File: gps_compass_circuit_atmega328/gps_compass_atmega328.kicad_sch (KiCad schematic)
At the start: 3 parts, among them U3 ATmega328P-A

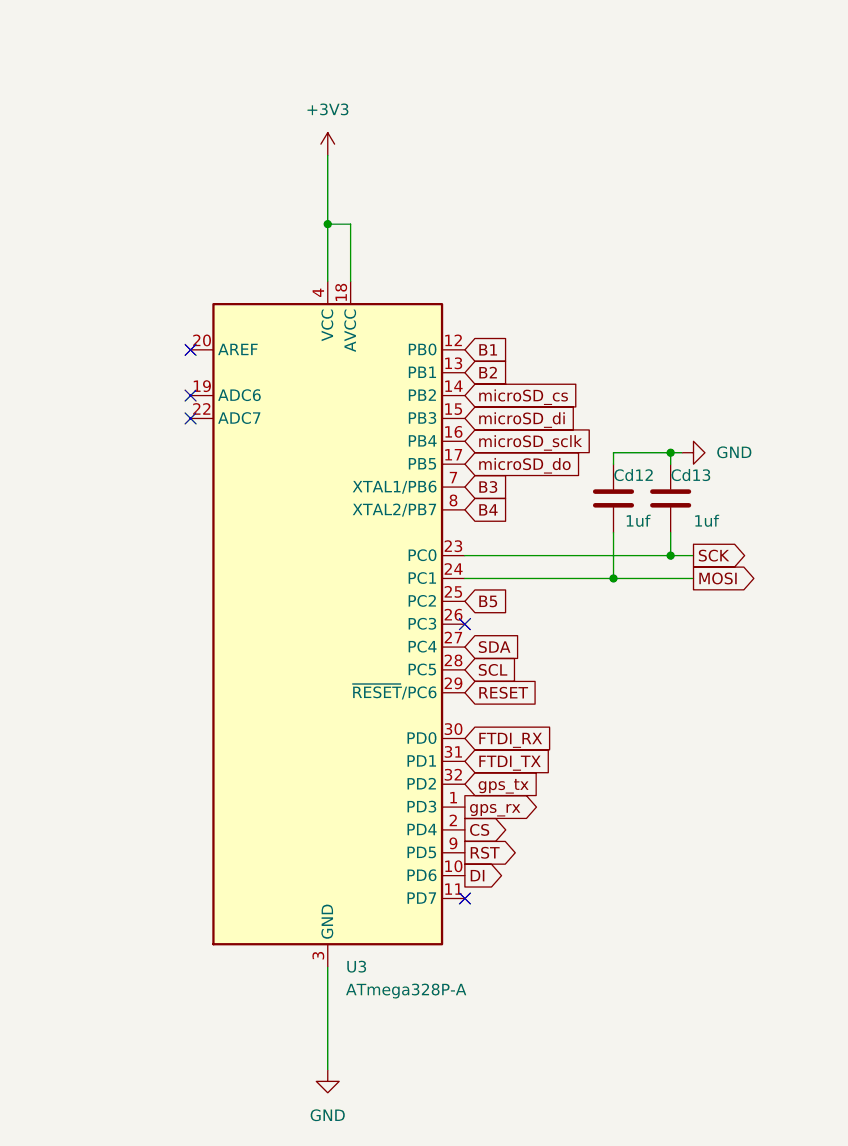
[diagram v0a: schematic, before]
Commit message: upd circuit
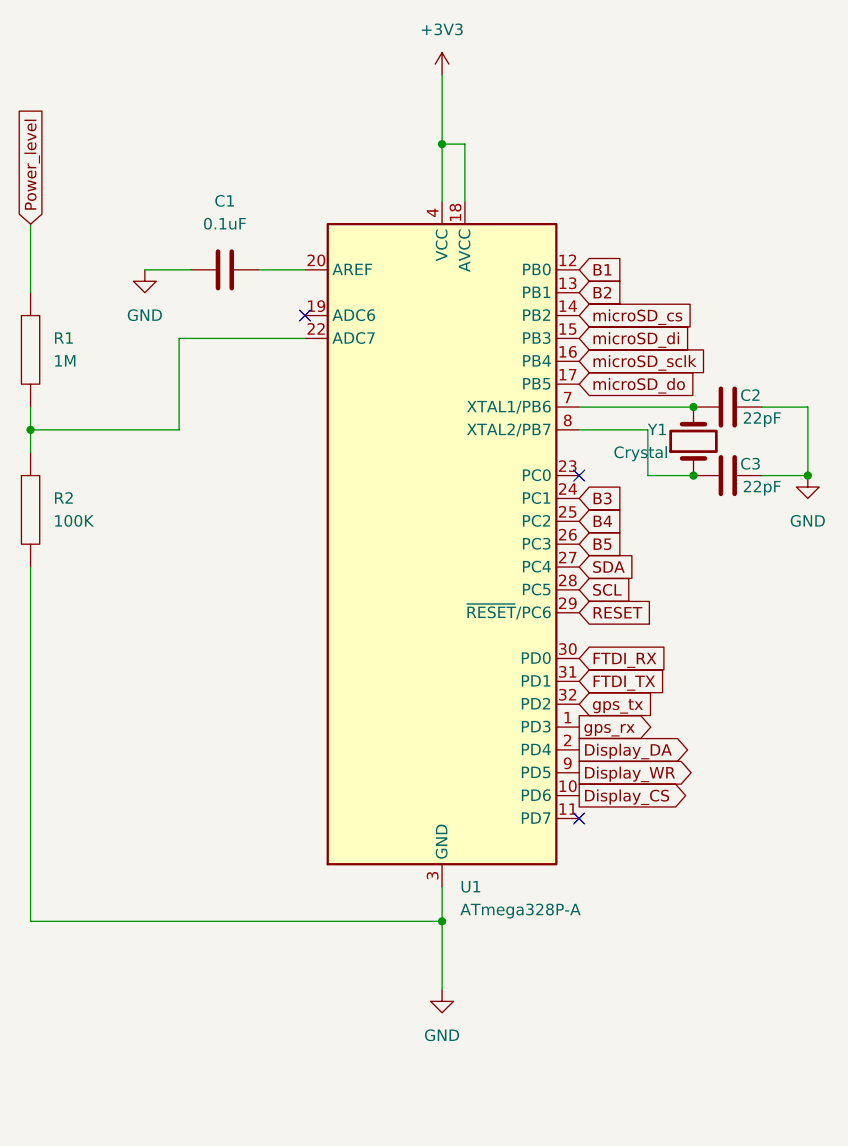
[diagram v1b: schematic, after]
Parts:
- removed Cd12, Cd13: 1uf, Capacitor_SMD:C_0603_1608Metric, symbol Device:C
- removed U3: ATmega328P-A, Package_QFP:TQFP-32_7x7mm_P0.8mm, symbol MCU_Microchip_ATmega:ATmega328P-A
- added C1: 0.1uF, Capacitor_SMD:C_0603_1608Metric, symbol Device:C
- added C2, C3: 22pF, Capacitor_SMD:C_0603_1608Metric, symbol Device:C
- added R1: 1M, Capacitor_SMD:C_0603_1608Metric, symbol pspice:R
- added R2: 100K, Capacitor_SMD:C_0603_1608Metric, symbol pspice:R
- added U1: ATmega328P-A, Package_QFP:TQFP-32_7x7mm_P0.8mm, symbol MCU_Microchip_ATmega:ATmega328P-A
- added Y1: Crystal, Crystal:Resonator-2Pin_W10.0mm_H5.0mm, symbol Device:Crystal
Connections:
- net +3V3: now also U1.18 (AVCC), U1.4 (VCC), U1.6 (VCC)
- net B1: now also U1.12 (PB0)
- net B2: now also U1.13 (PB1)
- net B3: now also U1.24 (PC1)
- net B4: now also U1.25 (PC2)
- net B5: now also U1.26 (PC3)
- net FTDI_RX: now also U1.30 (PD0)
- net FTDI_TX: now also U1.31 (PD1)
- net GND: now also C1.1, C2.2, C3.2, R2.2, U1.21 (GND), U1.3 (GND), U1.5 (GND)
- net RESET: now also U1.29 (~{RESET}/PC6)
- net SCL: now also U1.28 (PC5)
- net SDA: now also U1.27 (PC4)
- net gps_rx: now also U1.1 (PD3)
- net gps_tx: now also U1.32 (PD2)
- net microSD_cs: now also U1.14 (PB2)
- net microSD_di: now also U1.15 (PB3)
- net microSD_do: now also U1.17 (PB5)
- net microSD_sclk: now also U1.16 (PB4)
- new net: C3.1, U1.8 (XTAL2/PB7), Y1.1
- new net: C2.1, U1.7 (XTAL1/PB6), Y1.2
- new net: C1.2, U1.20 (AREF)
- new net: R1.2, R2.1, U1.22 (ADC7)
- new net Display_CS: U1.10 (PD6)
- new net Display_DA: U1.2 (PD4)
- new net Display_WR: U1.9 (PD5)
- new net Power_level: R1.1
- no-connect marks 5 -> 3
